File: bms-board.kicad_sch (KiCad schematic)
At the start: 1 part, among them U1 LTC6804-2

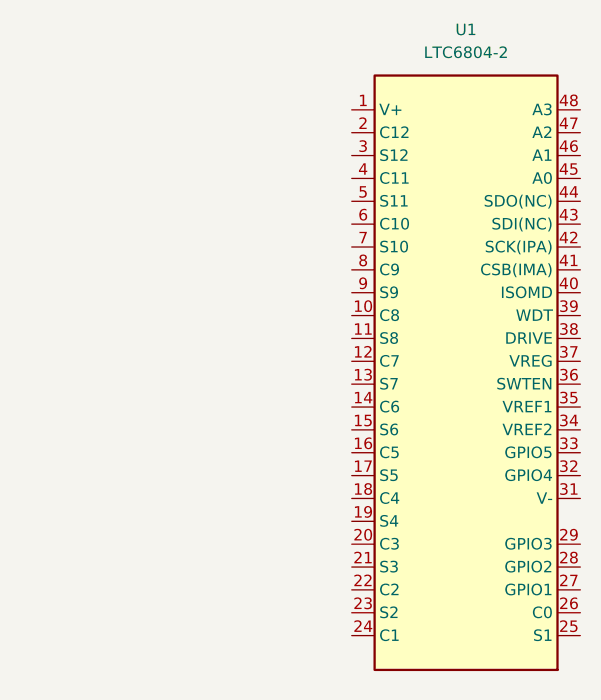
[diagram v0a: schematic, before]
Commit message: Merging new develop into new feature (#6)
* feat: add 6804-2 kicad symbol

* TEMPLATE: add pull request description template

* feat: add automated git flow setup script

* update feature/our-symbol-library branch to latest develop edition (#5)

* TEMPLATE: add pull request description template

* feat: add automated git flow setup script

* feat: a maybe working fixed wing schematic symbol library

* feat: add line to checkout dev branch when running setup script

* feat: fix FixedWing symbol library to include LTC6804-2

* refactor: verifying symbol library works, remove individual ltc6804-2 symbol

* feat: adding needed files

* feat: edit conflict in setup script

---------

Co-authored-by: Ephram Cola Jacquin <89238547+ephram2004@users.noreply.github.com>
Co-authored-by: Ephram Cola Jacquin <ecolajacquin@gmail.com>
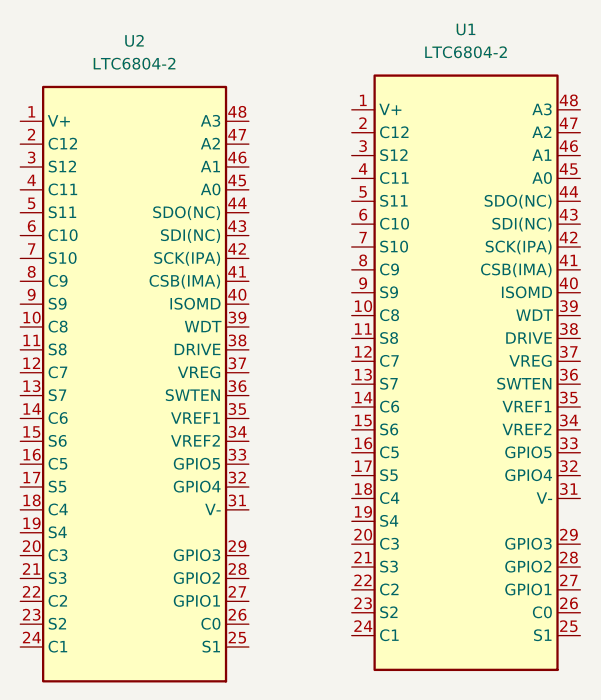
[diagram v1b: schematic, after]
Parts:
- added U2: LTC6804-2, Package_SO:SSOP-48_5.3x12.8mm_P0.5mm, symbol FixedWing:LTC6804-2
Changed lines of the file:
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@@
 (kicad_sch (version 20230121) (generator eeschema)
   (paper "A4")
+  (symbol (lib_id "FixedWing:LTC6804-2") (at 111.76 93.98 0) (unit 1)
+    (in_bom yes) (on_board yes) (dnp no) (fields_autoplaced)
+    (property "Reference" "U2" (at 111.76 55.88 0)
+      (effects (font (size 1.27 1.27)))
+    )
+    (property "Value" "LTC6804-2" (at 111.76 58.42 0)
+      (effects (font (size 1.27 1.27)))
+    )
+    (property "Footprint" "Package_SO:SSOP-48_5.3x12.8mm_P0.5mm" (at 111.76 132.08 0)
+      (effects (font (size 1.27 1.27)) hide)
+    )
+    (property "Datasheet" "https://www.analog.com/media/en/technical-documentation/data-sheets/680412fc.pdf" (at 114.3 57.15 0)
+      (effects (font (size 1.27 1.27)) hide)
+    )
+    (pin "44")
+    (pin "11")
+    (pin "12")
+    (pin "36")
+    (pin "37")
+    (pin "4")
+    (pin "14")
+    (pin "41")
+    (pin "10")
+    (pin "2")
+    (pin "22")
+    (pin "40")
+    (pin "46")
+    (pin "5")
+    (pin "29")
+    (pin "9")
+    (pin "24")
+    (pin "21")
+    (pin "31")
+    (pin "42")
+    (pin "47")
+    (pin "13")
+    (pin "3")
+    (pin "48")
+    (pin "6")
+    (pin "32")
+    (pin "34")
+    (pin "20")
+    (pin "8")
+    (pin "1")
+    (pin "28")
+    (pin "19")
+    (pin "26")
+    (pin "15")
+    (pin "38")
+    (pin "16")
+    (pin "35")
+    (pin "43")
+    (pin "33")
+    (pin "17")
+    (pin "18")
+    (pin "25")
+    (pin "45")
+    (pin "7")
+    (pin "23")
+    (pin "30")
+    (pin "27")
+    (pin "39")
+    (instances
+      (project "bms-board"
+        (path "/8a7831d1-a913-4f04-8780-225d2234b41d"
+          (reference "U2") (unit 1)
+        )
+      )
+    )
+  )
   (symbol (lib_id "Battery_Management:LTC6804-2") (at 148.59 92.71 0) (unit 1)
     (in_bom yes) (on_board yes) (dnp no) (fields_autoplaced)
